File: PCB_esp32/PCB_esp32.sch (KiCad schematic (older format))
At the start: 1 part

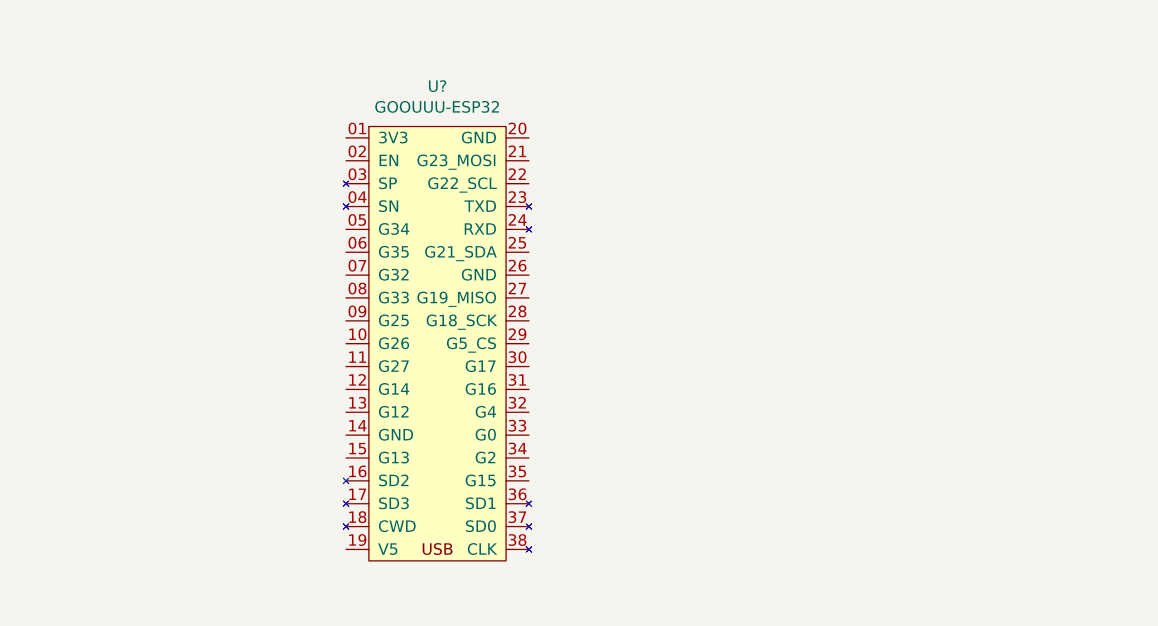
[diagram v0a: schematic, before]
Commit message: [PCB ESP32 e NRF]
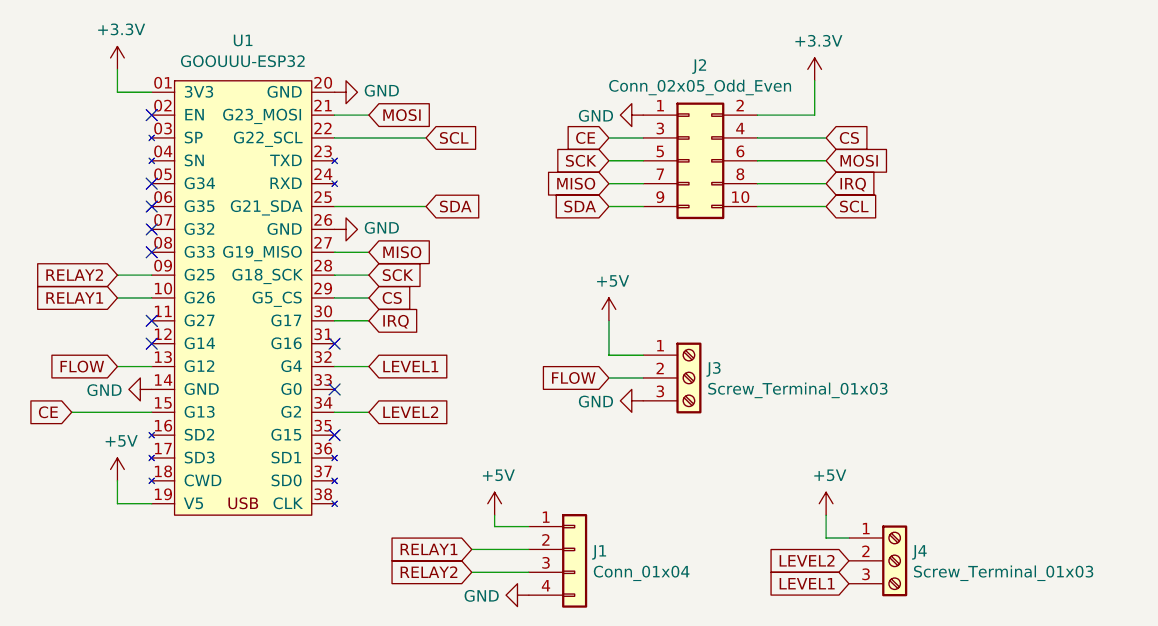
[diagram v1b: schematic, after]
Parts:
- removed U?: GOOUUU-ESP32, PI2_footprint:GOOUUU-ESP32, symbol PI2_Library:GOOUUU-ESP32
- added J1: Conn_01x04, Connector_PinHeader_2.54mm:PinHeader_1x04_P2.54mm_Vertical, symbol Connector_Generic:Conn_01x04
- added J2: Conn_02x05_Odd_Even, Connector_IDC:IDC-Header_2x05_P2.54mm_Vertical, symbol Connector_Generic:Conn_02x05_Odd_Even
- added J3, J4: Screw_Terminal_01x03, TerminalBlock_Philmore:TerminalBlock_Philmore_TB133_1x03_P5.00mm_Horizontal, symbol Connector:Screw_Terminal_01x03
- added U1: GOOUUU-ESP32, PI2_footprint:GOOUUU-ESP32, symbol PI2_Library:GOOUUU-ESP32
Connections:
- new net +3V3: J2.2 (Pin_2), U1.01 (3V3)
- new net +5V: J1.1 (Pin_1), J3.1 (Pin_1), J4.1 (Pin_1), U1.19 (V5)
- new net CE: J2.3 (Pin_3), U1.15 (G13)
- new net CS: J2.4 (Pin_4), U1.29 (G5_CS)
- new net FLOW: J3.2 (Pin_2), U1.13 (G12)
- new net GND: J1.4 (Pin_4), J2.1 (Pin_1), J3.3 (Pin_3), U1.14 (GND), U1.20 (GND), U1.26 (GND)
- new net IRQ: J2.8 (Pin_8), U1.30 (G17)
- new net LEVEL1: J4.3 (Pin_3), U1.32 (G4)
- new net LEVEL2: J4.2 (Pin_2), U1.34 (G2)
- new net MISO: J2.7 (Pin_7), U1.27 (G19_MISO)
- new net MOSI: J2.6 (Pin_6), U1.21 (G23_MOSI)
- new net RELAY1: J1.2 (Pin_2), U1.10 (G26)
- new net RELAY2: J1.3 (Pin_3), U1.09 (G25)
- new net SCK: J2.5 (Pin_5), U1.28 (G18_SCK)
- new net SCL: J2.10 (Pin_10), U1.22 (G22_SCL)
- new net SDA: J2.9 (Pin_9), U1.25 (G21_SDA)
- no-connect marks 0 -> 10
